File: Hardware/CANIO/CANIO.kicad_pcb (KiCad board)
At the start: 2 copper layers, 11 parts, among them J201 CAN, J202 CAN, U201 MCP25625-x-SS, Y201 16mHz

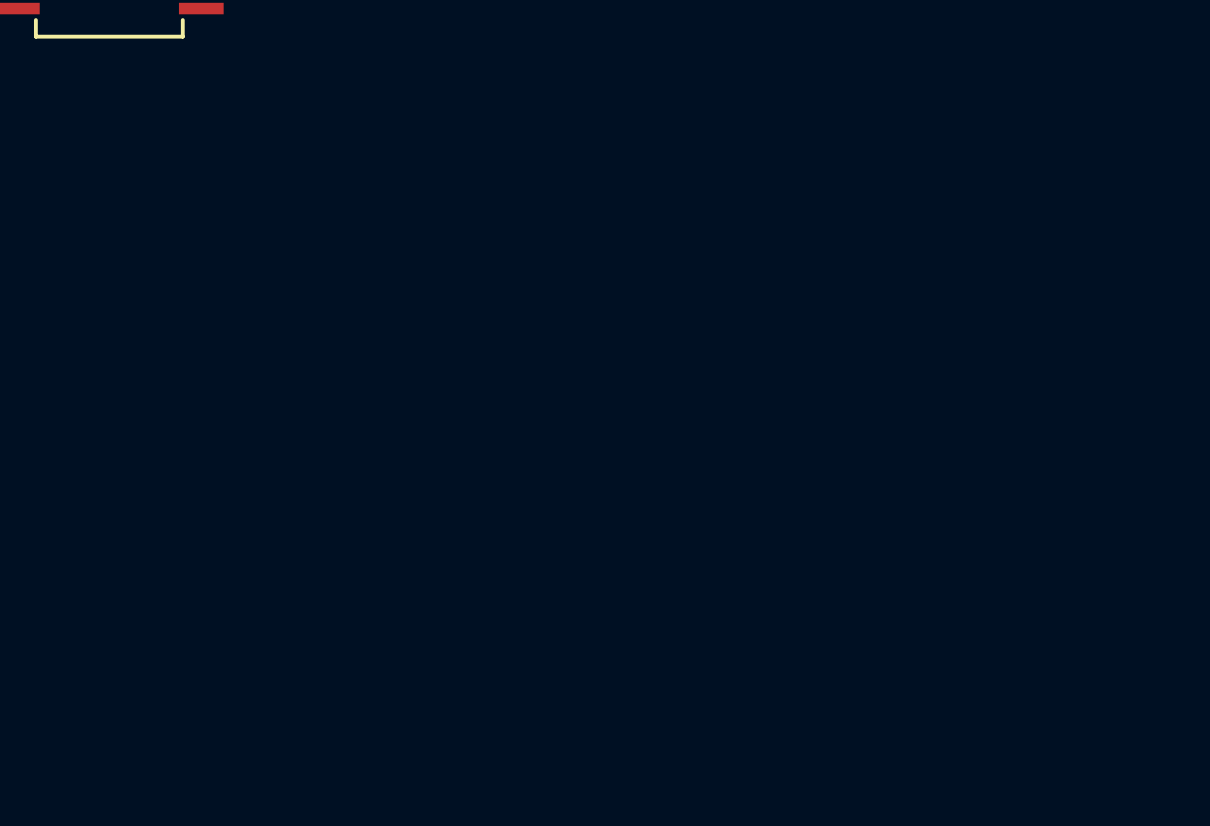
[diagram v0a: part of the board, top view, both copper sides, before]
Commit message: Add processor
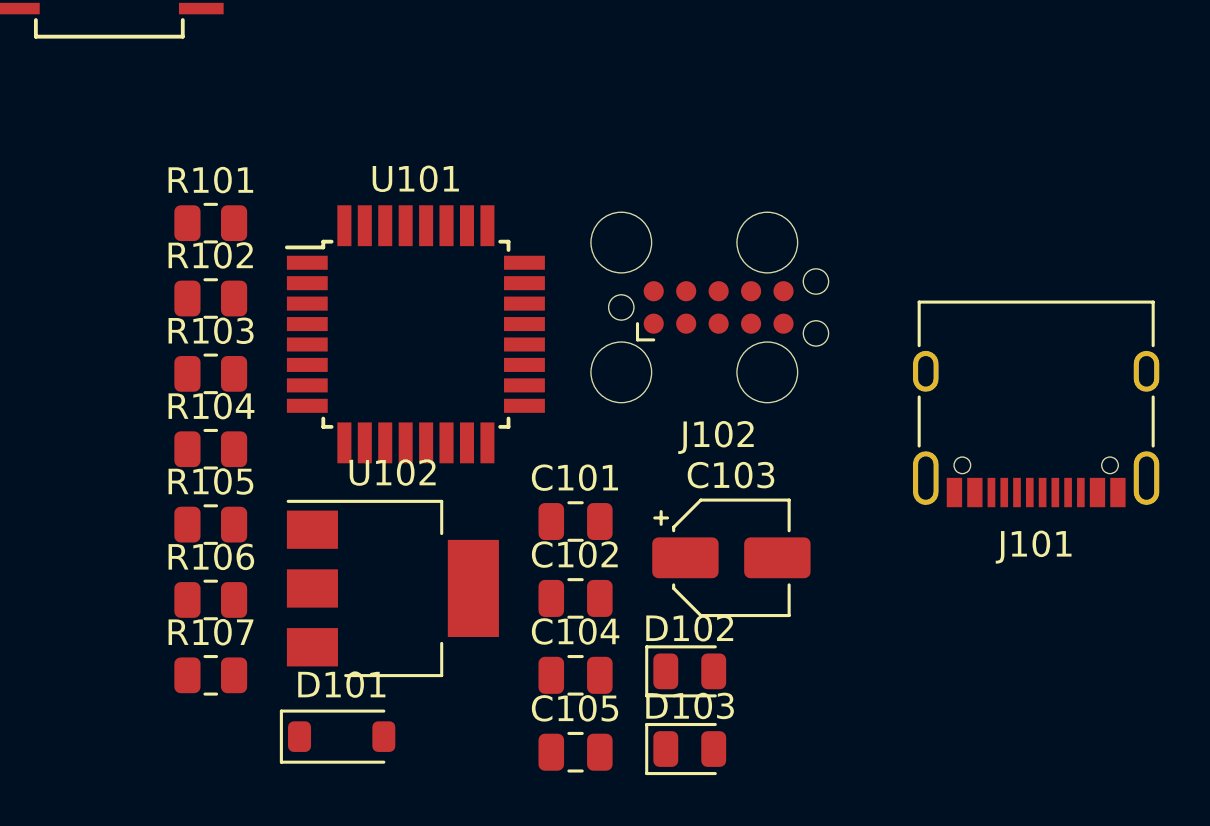
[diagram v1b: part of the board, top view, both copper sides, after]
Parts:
- added C101: 1u, Capacitor_SMD:C_0805_2012Metric, F.Cu at (31.6, 9.58)
- added C102: 100nF, Capacitor_SMD:C_0805_2012Metric, F.Cu at (31.6, 12.6)
- added C103: 10uf, Capacitor_SMD:CP_Elec_4x3, F.Cu at (37.8, 11.0)
- added C104: 100nF, Capacitor_SMD:C_0805_2012Metric, F.Cu at (31.6, 15.6)
- added C105: 1uF, Capacitor_SMD:C_0805_2012Metric, F.Cu at (31.6, 18.6)
- added D101: MBR0520LT, Diode_SMD:D_SOD-123, F.Cu at (22.5, 18.0)
- added D102: STAT, LED_SMD:LED_0805_2012Metric, F.Cu at (36.1, 15.4)
- added D103: PWR, LED_SMD:LED_0805_2012Metric, F.Cu at (36.1, 18.5)
- added J101: USBC, KenwoodFox:USB_C_Receptacle_XKB_U262-16XN-4BVC11_Full_Pads, F.Cu at (49.7, 4.78)
- added J102: Tag Connect, Connector:Tag-Connect_TC2050-IDC-FP_2x05_P1.27mm_Vertical, F.Cu at (37.2, 1.20)
- added R101: 22R, Resistor_SMD:R_0805_2012Metric, F.Cu at (17.4, -2.10)
- added R102: 22R, Resistor_SMD:R_0805_2012Metric, F.Cu at (17.4, 0.85)
- added R103: 10k, Resistor_SMD:R_0805_2012Metric, F.Cu at (17.4, 3.80)
- added R104: 5K1, Resistor_SMD:R_0805_2012Metric, F.Cu at (17.4, 6.75)
- added R105: 5K1, Resistor_SMD:R_0805_2012Metric, F.Cu at (17.4, 9.70)
- added R106: 1K, Resistor_SMD:R_0805_2012Metric, F.Cu at (17.4, 12.7)
- added R107: 1K, Resistor_SMD:R_0805_2012Metric, F.Cu at (17.4, 15.6)
- added U101: ATmega16U2, Package_QFP:TQFP-32_7x7mm_P0.8mm, F.Cu at (25.4, 2.25)
- added U102: LM1117MP-5.0, Package_TO_SOT_SMD:SOT-223-3_TabPin2, F.Cu at (24.5, 12.2)
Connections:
- net Net-(U201-STBY) renamed /CANBUS/STBY
- U201 pad 13: unconnected-(U201-~{INT}-Pad13) -> /CANBUS/INT
- U201 pad 22: /CANBUS/CLKOUT -> /CLKOUT

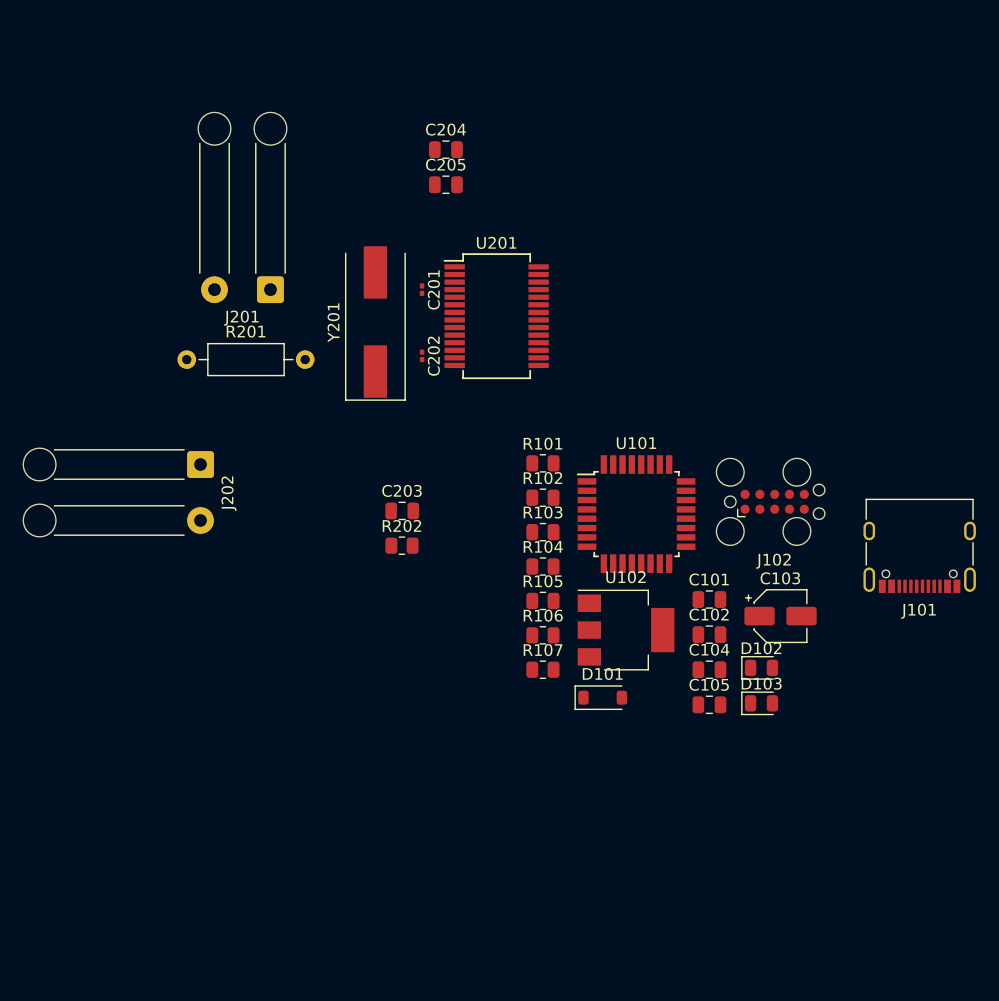
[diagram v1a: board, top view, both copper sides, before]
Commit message: Bump
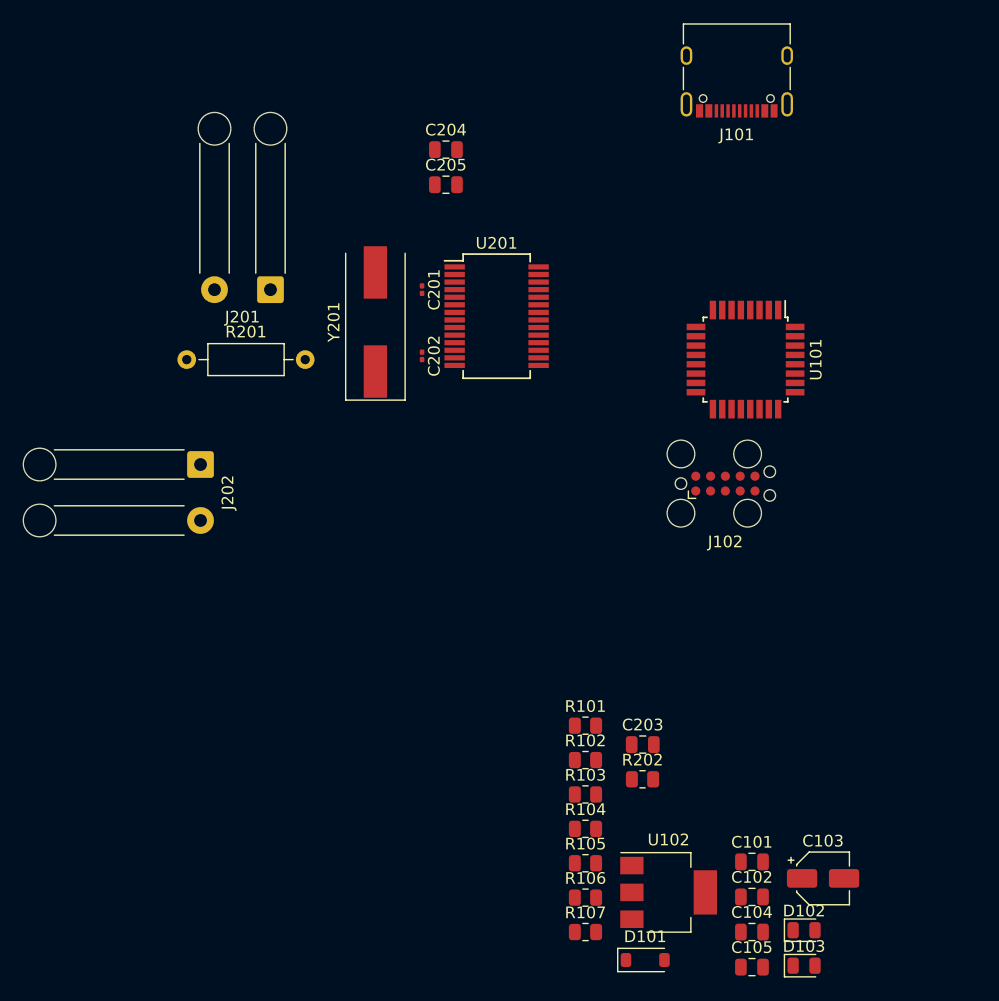
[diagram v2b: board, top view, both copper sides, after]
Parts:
- moved J101 43.7 mm to (34.0, -36.0)
- moved C203 28.8 mm to (25.9, 22.0)
- moved R202 28.8 mm to (25.9, 25.0)
- moved C102 22.8 mm to (35.3, 35.1)
- moved D102 22.8 mm to (39.8, 37.9)
- moved D103 22.8 mm to (39.8, 41.0)
- moved R105 22.8 mm to (21.0, 32.2)
- moved U102 22.8 mm to (28.1, 34.7)
- moved C101 22.8 mm to (35.3, 32.1)
- moved C103 22.8 mm to (41.4, 33.5)
- moved C104 22.8 mm to (35.3, 38.1)
- moved C105 22.8 mm to (35.3, 41.1)
- moved D101 22.8 mm to (26.1, 40.5)
- moved R101 22.8 mm to (21.0, 20.4)
- moved R102 22.8 mm to (21.0, 23.4)
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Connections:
- U201 pad 14: /CANBUS/SCK -> /ICSP_SCK
- U201 pad 15: /CANBUS/SI -> /ICSP_MOSI
- U201 pad 16: /CANBUS/SO -> /ICSP_MISO
